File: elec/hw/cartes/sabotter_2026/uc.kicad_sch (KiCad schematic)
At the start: 39 parts, among them J3 USB4120-03-C, SW1 PTS525 SK15 SMTR2 LFS, SW2 SLW-713515-2A-SMT-TR, SW3 DSIC01LSGER, U3 ESP32-S3-WROOM-1

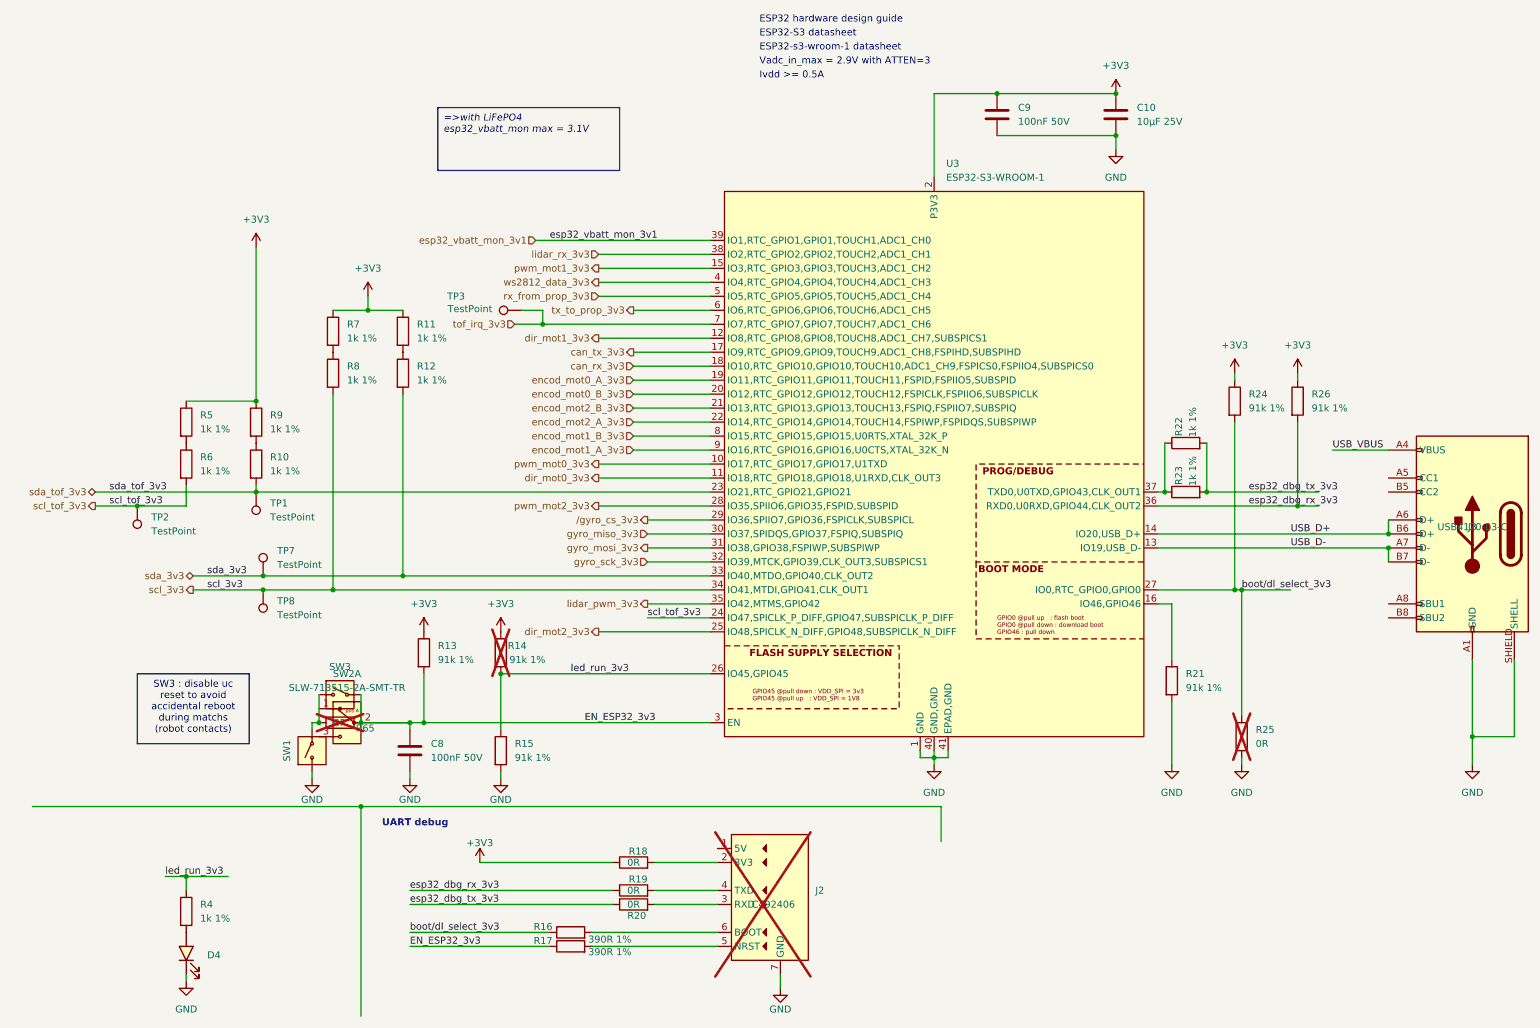
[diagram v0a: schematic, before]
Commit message: sabotter corrected after review
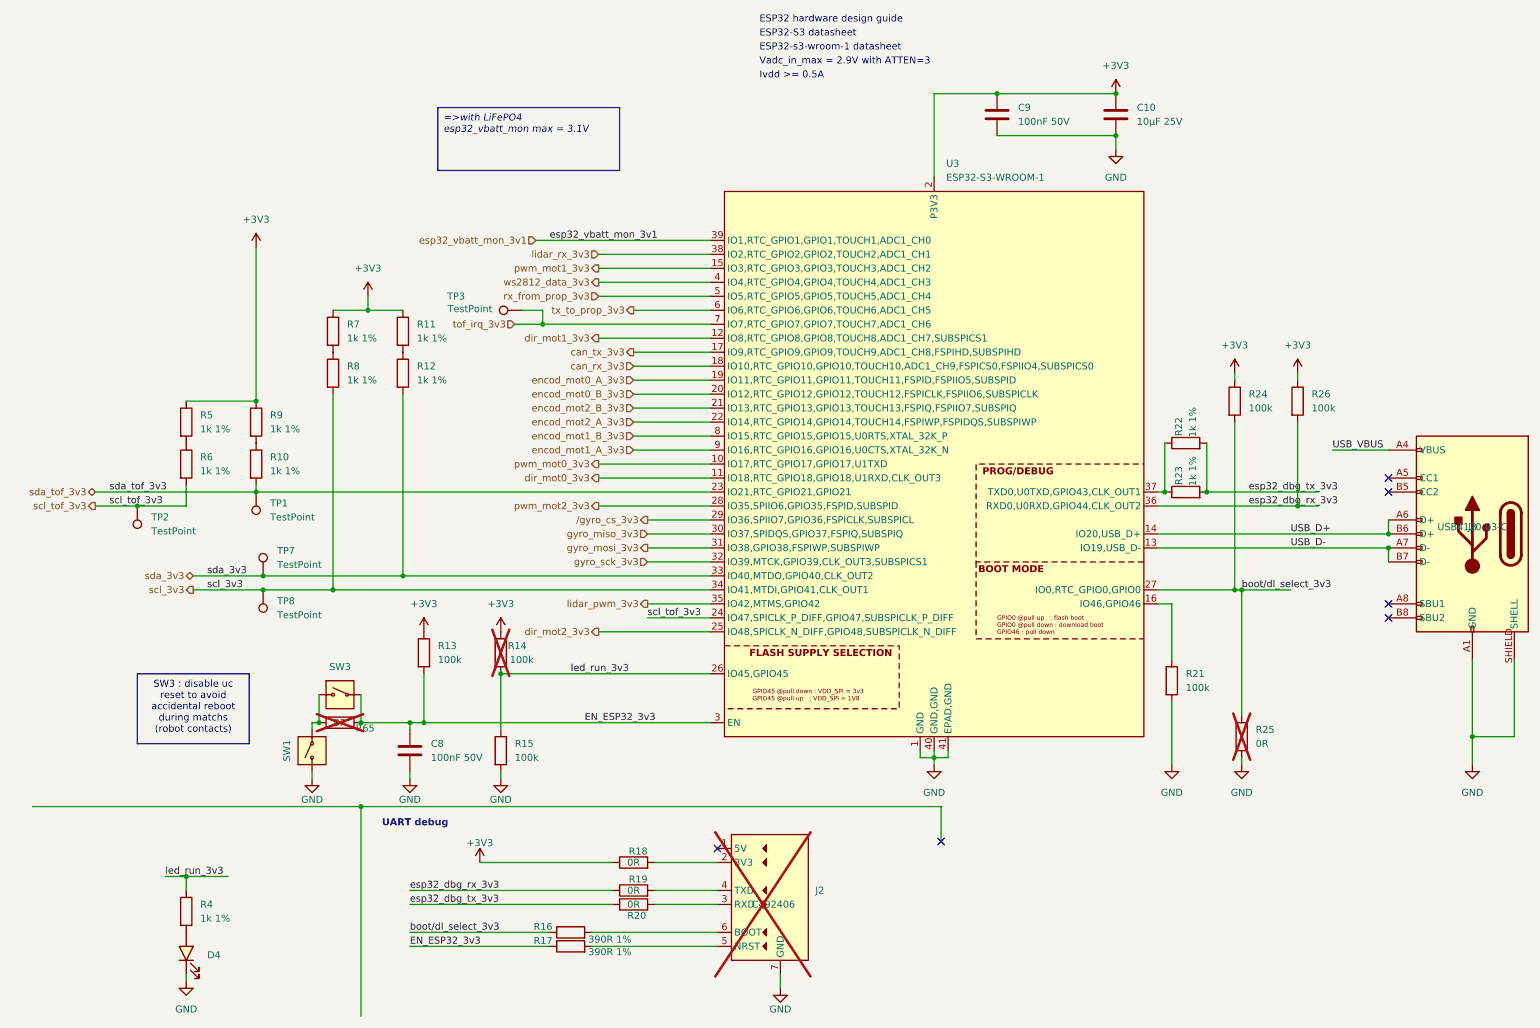
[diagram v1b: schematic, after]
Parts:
- removed SW2: SLW-713515-2A-SMT-TR, cocotter_others:SLW-713515-2A-SMT-TR, symbol cocotter_connectors:SLW-713515-2A-SMT-TR
- R13, R14, R15, R21, R24, R26: value 91k 1% -> 100k; symbol cocotter_resistors:R_91k_0603_1% -> cocotter_resistors:R_100k_0603_1%; JLCPCB Part # C23265 -> C25803; Specification 91k 0603 1% 100mW -> 100k 0603 1% 100mW; mouser (none) -> 603-RC0603FR-10100KL
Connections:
- no-connect marks 0 -> 6
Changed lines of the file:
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@@
 		(color 0 0 0 0)
 	)
+	(no_connect
+		(at 257.81 99.06)
+	)
+	(no_connect
+		(at 257.81 124.46)
+	)
+	(no_connect
+		(at 135.89 166.37)
+	)
+	(no_connect
+		(at 257.81 101.6)
+	)
+	(no_connect
+		(at 176.53 165.1)
+	)
+	(no_connect
+		(at 257.81 121.92)
+	)
 	(wire
 		(pts
@@
 	(wire
 		(pts
-			(xy 73.66 143.51) (xy 80.01 143.51)
-		)
-		(stroke
-			(width 0)
-			(type default)
-		)
-	)
-	(wire
-		(pts
 			(xy 231.14 149.86) (xy 231.14 151.13)
 		)
@@
 	)
 	(symbol
-		(lib_id "cocotter_resistors:R_91k_0603_1%")
+		(lib_id "cocotter_resistors:R_100k_0603_1%")
 		(at 229.87 85.09 0)
 		(unit 1)
@@
 			)
 		)
-		(property "Value" "91k 1%"
+		(property "Value" "100k"
 			(at 232.41 86.3599 0)
 			(effects
@@
 			)
 		)
-		(property "Specification" "91k 0603 1% 100mW"
+		(property "Specification" "100k 0603 1% 100mW"
 			(at 229.87 85.09 0)
 			(effects
@@
 			)
 		)
-		(property "mouser" ""
+		(property "mouser" "603-RC0603FR-10100KL"
 			(at 229.87 85.09 0)
 			(effects
@@
 			)
 		)
-		(property "JLCPCB Part #" "C23265"
+		(property "JLCPCB Part #" "C25803"
 			(at 229.87 85.09 0)
 			(effects
@@
 	)
 	(symbol
-		(lib_id "cocotter_resistors:R_91k_0603_1%")
+		(lib_id "cocotter_resistors:R_100k_0603_1%")
 		(at 82.55 130.81 0)
 		(unit 1)
@@
 			)
 		)
-		(property "Value" "91k 1%"
+		(property "Value" "100k"
 			(at 85.09 132.0799 0)
 			(effects
@@
 			)
 		)
-		(property "Specification" "91k 0603 1% 100mW"
+		(property "Specification" "100k 0603 1% 100mW"
 			(at 82.55 130.81 0)
 			(effects
@@
 			)
 		)
-		(property "mouser" ""
+		(property "mouser" "603-RC0603FR-10100KL"
 			(at 82.55 130.81 0)
 			(effects
@@
 			)
 		)
-		(property "JLCPCB Part #" "C23265"
+		(property "JLCPCB Part #" "C25803"
 			(at 82.55 130.81 0)
 			(effects
@@
 	)
 	(symbol
-		(lib_id "cocotter_resistors:R_91k_0603_1%")
+		(lib_id "cocotter_resistors:R_100k_0603_1%")
 		(at 241.3 85.09 0)
 		(unit 1)
@@
 			)
 		)
-		(property "Value" "91k 1%"
+		(property "Value" "100k"
 			(at 243.84 86.3599 0)
 			(effects
@@
 			)
 		)
-		(property "Specification" "91k 0603 1% 100mW"
+		(property "Specification" "100k 0603 1% 100mW"
 			(at 241.3 85.09 0)
 			(effects
@@
 			)
 		)
-		(property "mouser" ""
+		(property "mouser" "603-RC0603FR-10100KL"
 			(at 241.3 85.09 0)
 			(effects
@@
 			)
 		)
-		(property "JLCPCB Part #" "C23265"
+		(property "JLCPCB Part #" "C25803"
 			(at 241.3 85.09 0)
 			(effects
@@
 	)
 	(symbol
-		(lib_id "cocotter_resistors:R_91k_0603_1%")
+		(lib_id "cocotter_resistors:R_100k_0603_1%")
 		(at 96.52 130.81 0)
 		(unit 1)
@@
 			)
 		)
-		(property "Value" "91k 1%"
-			(at 101.346 132.08 0)
+		(property "Value" "100k"
+			(at 100.33 132.08 0)
 			(effects
 				(font
@@
 			)
 		)
-		(property "Specification" "91k 0603 1% 100mW"
+		(property "Specification" "100k 0603 1% 100mW"
 			(at 96.52 130.81 0)
 			(effects
@@
 			)
 		)
-		(property "mouser" ""
+		(property "mouser" "603-RC0603FR-10100KL"
 			(at 96.52 130.81 0)
 			(effects
@@
 			)
 		)
-		(property "JLCPCB Part #" "C23265"
+		(property "JLCPCB Part #" "C25803"
 			(at 96.52 130.81 0)
 			(effects
@@
 	)
 	(symbol
-		(lib_id "cocotter_resistors:R_91k_0603_1%")
+		(lib_id "cocotter_resistors:R_100k_0603_1%")
 		(at 96.52 148.59 0)
 		(unit 1)
@@
 			)
 		)
-		(property "Value" "91k 1%"
+		(property "Value" "100k"
 			(at 99.06 149.8599 0)
 			(effects
@@
 			)
 		)
-		(property "Specification" "91k 0603 1% 100mW"
+		(property "Specification" "100k 0603 1% 100mW"
 			(at 96.52 148.59 0)
 			(effects
@@
 			)
 		)
-		(property "mouser" ""
+		(property "mouser" "603-RC0603FR-10100KL"
 			(at 96.52 148.59 0)
 			(effects
@@
 			)
 		)
-		(property "JLCPCB Part #" "C23265"
+		(property "JLCPCB Part #" "C25803"
 			(at 96.52 148.59 0)
 			(effects
@@
 	)
 	(symbol
-		(lib_id "cocotter_connectors:SLW-713515-2A-SMT-TR ")
-		(at 68.58 143.51 0)
-		(unit 1)
-		(exclude_from_sim no)
-		(in_bom yes)
-		(on_board yes)
-		(dnp no)
-		(fields_autoplaced yes)
-		(property "Reference" "SW2"
-			(at 68.58 134.62 0)
-			(effects
-				(font
-					(size 1.27 1.27)
-				)
-			)
-		)
-		(property "Value" "SLW-713515-2A-SMT-TR"
-			(at 68.58 137.16 0)
-			(effects
-				(font
-					(size 1.27 1.27)
-				)
-			)
-		)
-		(property "Footprint" "cocotter_others:SLW-713515-2A-SMT-TR"
-			(at 68.58 143.51 0)
-			(effects
-				(font
-					(size 1.27 1.27)
-				)
-				(hide yes)
-			)
-		)
-		(property "Datasheet" "https://www.sameskydevices.com/product/resource/slw-713515-2a-smt-tr.pdf"
-			(at 68.58 148.59 0)
-			(effects
-				(font
-					(size 1.27 1.27)
-				)
-				(hide yes)
-			)
-		)
-		(property "Description" "50mA max, 12Vdc, 10000 cycles"
-			(at 68.58 143.51 0)
-			(effects
-				(font
-					(size 1.27 1.27)
-				)
-				(hide yes)
-			)
-		)
-		(property "JLCPCB Part #" "C2858291"
-			(at 67.31 148.59 0)
-			(effects
-				(font
-					(size 1.27 1.27)
-				)
-				(hide yes)
-			)
-		)
-		(pin "2"
-		)
-		(pin "1"
-		)
-		(pin "3"
-		)
-		(pin "6"
-		)
-		(pin "4"
-		)
-		(pin "5"
-		)
-		(instances
-			(project ""
-				(path "/c1bd5504-d0b2-4cc3-94d1-261f58816249/0627c134-32e1-430c-bbd1-677b8ecf53c1"
-					(reference "SW2")
-					(unit 1)
-				)
-			)
-		)
-	)
-	(symbol
 		(lib_id "cocotter_resistors:R_0R_0603")
 		(at 120.65 173.99 90)
@@
 	)
 	(symbol
-		(lib_id "cocotter_resistors:R_91k_0603_1%")
+		(lib_id "cocotter_resistors:R_100k_0603_1%")
 		(at 218.44 135.89 0)
 		(unit 1)
@@
 			)
 		)
-		(property "Value" "91k 1%"
+		(property "Value" "100k"
 			(at 220.98 137.1599 0)
 			(effects
@@
 			)
 		)
-		(property "Specification" "91k 0603 1% 100mW"
+		(property "Specification" "100k 0603 1% 100mW"
 			(at 218.44 135.89 0)
 			(effects
@@
 			)
 		)
-		(property "mouser" ""
+		(property "mouser" "603-RC0603FR-10100KL"
 			(at 218.44 135.89 0)
 			(effects
@@
 			)
 		)
-		(property "JLCPCB Part #" "C23265"
+		(property "JLCPCB Part #" "C25803"
 			(at 218.44 135.89 0)
 			(effects
